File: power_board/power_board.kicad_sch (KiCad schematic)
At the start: 8 parts, among them CN1 XT90PW-M.G.Y, CN2 XT60PW-M, U1 MR60PW-M.G.B

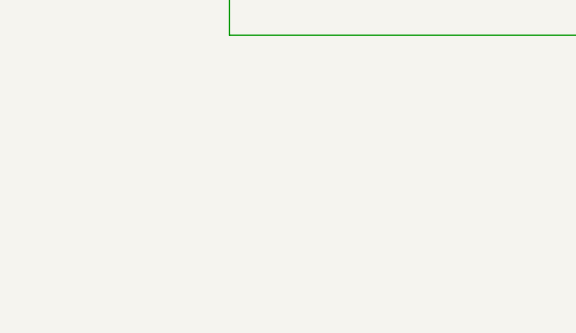
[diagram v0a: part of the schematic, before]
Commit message: Add JLCJLCJLCJLC
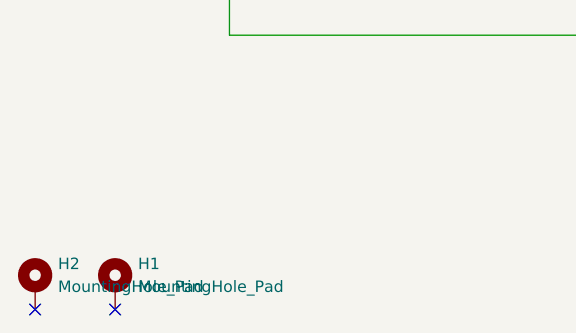
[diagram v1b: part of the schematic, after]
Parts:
- added H1, H2: MountingHole_Pad, MountingHole:MountingHole_4.3mm_M4_Pad_Via, symbol Mechanical:MountingHole_Pad
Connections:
- no-connect marks 6 -> 8
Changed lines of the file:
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@@
+	)
+	(no_connect
+		(at 46.99 177.8)
 	)
 	(no_connect
@@
 	)
 	(no_connect
+		(at 38.1 177.8)
+	)
+	(no_connect
 		(at 209.55 74.93)
 	)
@@
 			(width 0)
 			(type default)
+		)
+	)
+	(symbol
+		(lib_id "Mechanical:MountingHole_Pad")
+		(at 46.99 175.26 0)
+		(unit 1)
+		(exclude_from_sim no)
+		(in_bom no)
+		(on_board yes)
+		(dnp no)
+		(fields_autoplaced yes)
+		(property "Reference" "H1"
+			(at 49.53 172.7199 0)
+			(effects
+				(font
+					(size 1.27 1.27)
+				)
+				(justify left)
+			)
+		)
+		(property "Value" "MountingHole_Pad"
+			(at 49.53 175.2599 0)
+			(effects
+				(font
+					(size 1.27 1.27)
+				)
+				(justify left)
+			)
+		)
+		(property "Footprint" "MountingHole:MountingHole_4.3mm_M4_Pad_Via"
+			(at 46.99 175.26 0)
+			(effects
+				(font
+					(size 1.27 1.27)
+				)
+				(hide yes)
+			)
+		)
+		(property "Datasheet" "~"
+			(at 46.99 175.26 0)
+			(effects
+				(font
+					(size 1.27 1.27)
+				)
+				(hide yes)
+			)
+		)
+		(property "Description" "Mounting Hole with connection"
+			(at 46.99 175.26 0)
+			(effects
+				(font
+					(size 1.27 1.27)
+				)
+				(hide yes)
+			)
+		)
+		(pin "1"
+		)
+		(instances
+			(project ""
+				(path "/c786dd1f-c97f-4c1e-a27a-ac5828b3c50c"
+					(reference "H1")
+					(unit 1)
+				)
+			)
 		)
 	)
@@
 					(unit 1)
 				)
+			)
+		)
+	)
+	(symbol
+		(lib_id "Mechanical:MountingHole_Pad")
+		(at 38.1 175.26 0)
+		(unit 1)
+		(exclude_from_sim no)
+		(in_bom no)
+		(on_board yes)
+		(dnp no)
+		(fields_autoplaced yes)
+		(property "Reference" "H2"
+			(at 40.64 172.7199 0)
+			(effects
+				(font
+					(size 1.27 1.27)
+				)
+				(justify left)
+			)
+		)
+		(property "Value" "MountingHole_Pad"
+			(at 40.64 175.2599 0)
+			(effects
+				(font
+					(size 1.27 1.27)
+				)
+				(justify left)
+			)
+		)
+		(property "Footprint" "MountingHole:MountingHole_4.3mm_M4_Pad_Via"
+			(at 38.1 175.26 0)
+			(effects
+				(font
+					(size 1.27 1.27)
+				)
+				(hide yes)
+			)
+		)
+		(property "Datasheet" "~"
+			(at 38.1 175.26 0)
+			(effects
+				(font
+					(size 1.27 1.27)
+				)
+				(hide yes)
+			)
+		)
+		(property "Description" "Mounting Hole with connection"
+			(at 38.1 175.26 0)
+			(effects
+				(font
+					(size 1.27 1.27)
+				)
+				(hide yes)
+			)
+		)
+		(pin "1"
+		)
+		(instances
+			(project "power_board"
+				(path "/c786dd1f-c97f-4c1e-a27a-ac5828b3c50c"
+					(reference "H2")
+					(unit 1)
+				)
